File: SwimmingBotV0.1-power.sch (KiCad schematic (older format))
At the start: 17 parts, among them U1 LT3470A, U10 TPS6216X

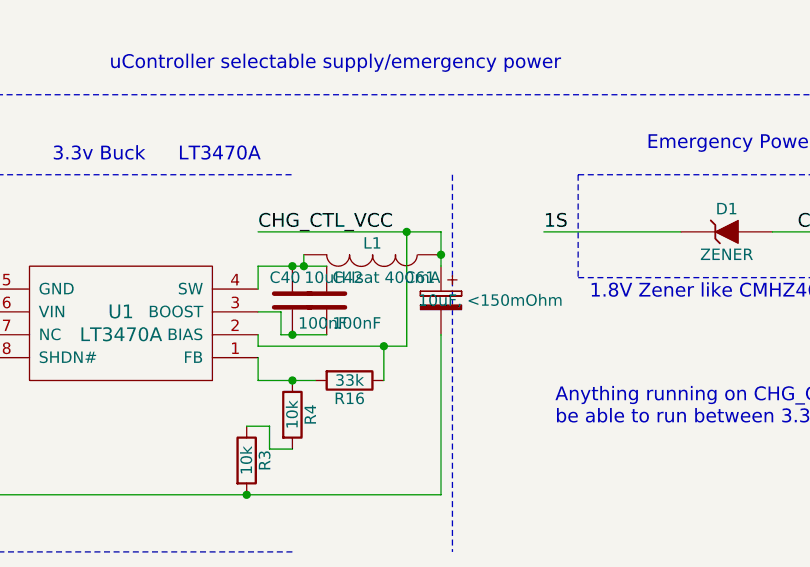
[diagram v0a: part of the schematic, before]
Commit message: hoh, working on power stuffs now
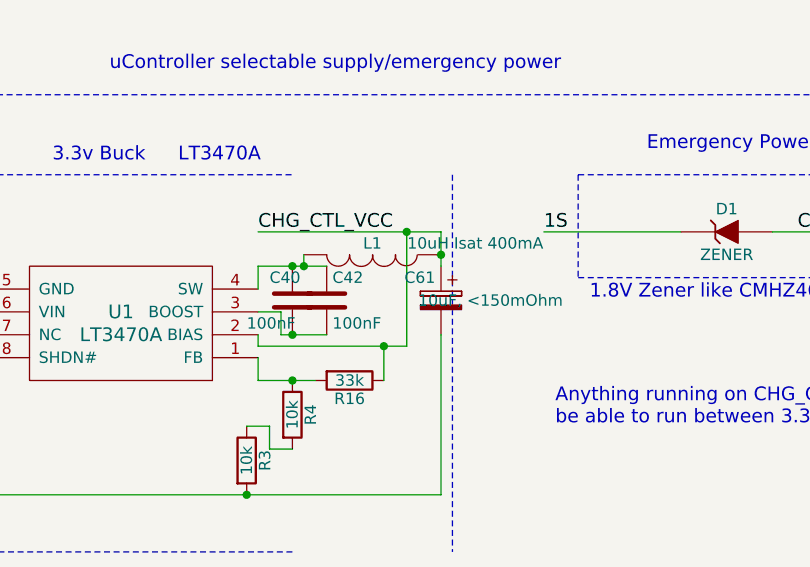
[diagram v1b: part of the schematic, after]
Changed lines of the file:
@@
 $Descr A4 11693 8268
 encoding utf-8
-Sheet 3 8
+Sheet 2 8
 Title ""
 Date ""
@@
 P 7850 3950
 F 0 "L1" V 7800 3950 50  0000 C CNN
-F 1 "10uH Isat 400mA" V 7950 3950 50  0000 C CNN
+F 1 "10uH Isat 400mA" V 7800 4400 50  0000 C CNN
 F 2 "Resistors_SMD:R_1210" H 7850 3950 50  0001 C CNN
 F 3 "" H 7850 3950 50  0000 C CNN
@@
 P 7500 4150
 F 0 "C40" H 7400 4250 50  0000 L CNN
-F 1 "100nF" H 7525 4050 50  0000 L CNN
+F 1 "100nF" H 7300 4050 50  0000 L CNN
 F 2 "Capacitors_SMD:C_0402" H 7538 4000 50  0001 C CNN
 F 3 "" H 7500 4150 50  0000 C CNN
